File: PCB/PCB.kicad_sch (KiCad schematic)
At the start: 417 parts, among them J2 Conn_OLED_I2C, U1 74AHCT125

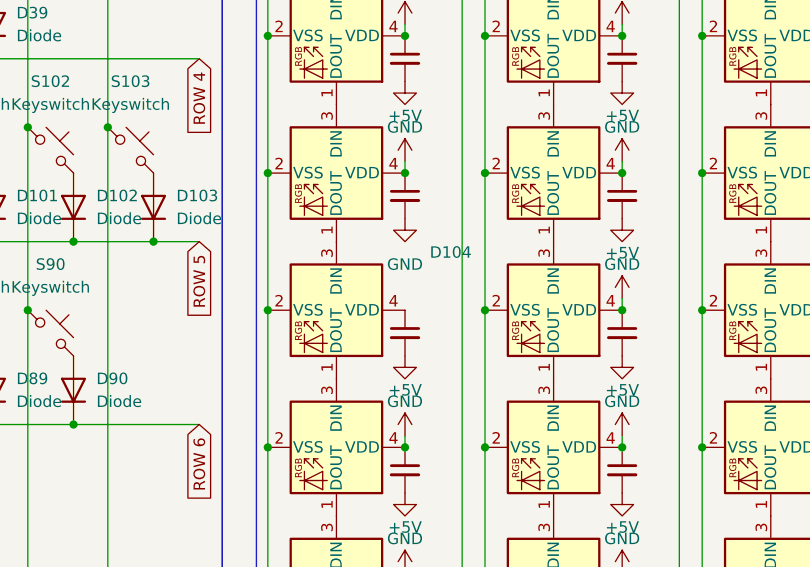
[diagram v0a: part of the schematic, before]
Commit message: did most of the wiring
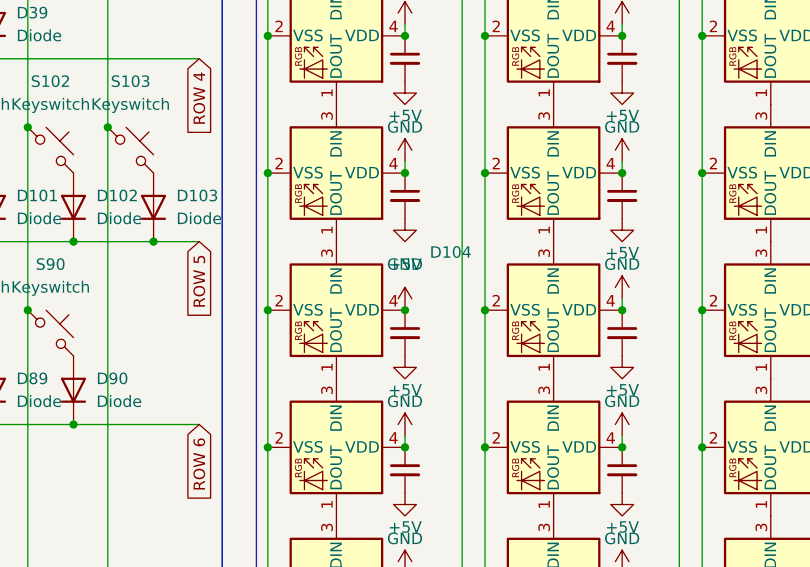
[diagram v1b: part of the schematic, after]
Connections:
- net +5V: now also C94.1, D104.4 (VDD)
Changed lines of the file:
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@@
 	)
 	(junction
+		(at 167.64 149.86)
+		(diameter 0)
+		(color 0 0 0 0)
+	)
+	(junction
 		(at 248.92 241.3)
 		(diameter 0)
@@
 					(unit 1)
 				)
+			)
+		)
+	)
+	(symbol
+		(lib_id "power:+5V")
+		(at 167.64 149.86 0)
+		(unit 1)
+		(exclude_from_sim no)
+		(in_bom yes)
+		(on_board yes)
+		(dnp no)
+		(fields_autoplaced yes)
+		(property "Reference" "#PWR0222"
+			(at 167.64 153.67 0)
+			(effects
+				(font
+					(size 1.27 1.27)
+				)
+				(hide yes)
+			)
+		)
+		(property "Value" "+5V"
+			(at 167.64 144.78 0)
+			(effects
+				(font
+					(size 1.27 1.27)
+				)
+			)
+		)
+		(property "Footprint" ""
+			(at 167.64 149.86 0)
+			(effects
+				(font
+					(size 1.27 1.27)
+				)
+				(hide yes)
+			)
+		)
+		(property "Datasheet" ""
+			(at 167.64 149.86 0)
+			(effects
+				(font
+					(size 1.27 1.27)
+				)
+				(hide yes)
+			)
+		)
+		(property "Description" "Power symbol creates a global label with name \"+5V\""
+			(at 167.64 149.86 0)
+			(effects
+				(font
+					(size 1.27 1.27)
+				)
+				(hide yes)
+			)
+		)
+		(pin "1"
+		)
+		(instances
+			(project "PCB"
+				(path "/9eec8c31-e2e7-4ce8-a19c-313dbd6669b7"
+					(reference "#PWR0222")
+					(unit 1)
+				)
